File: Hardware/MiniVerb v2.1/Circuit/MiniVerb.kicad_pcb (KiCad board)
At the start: 2 copper layers, 47.9 x 128.5 mm, 52 parts, among them J1 IDC_2x05, U1 TL074, U2 LM4040DBZ-10, U3 MCP6001-OT

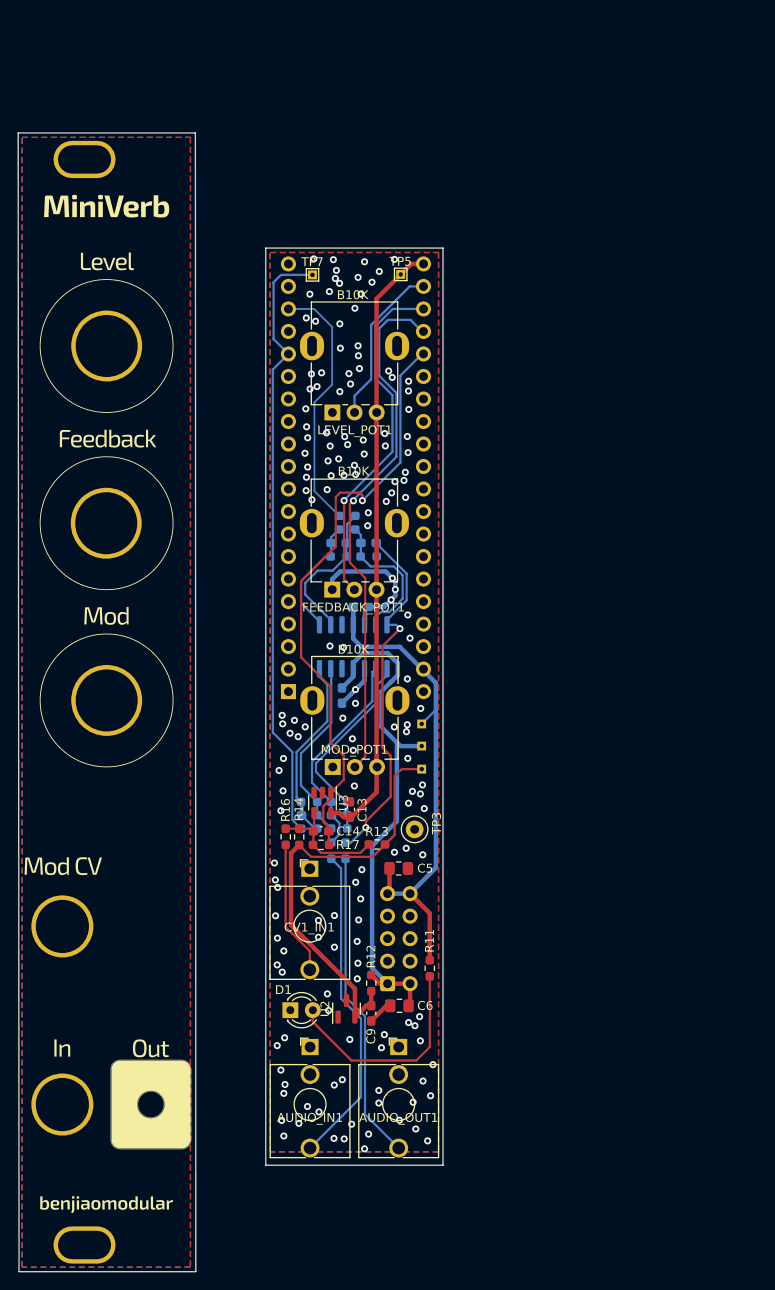
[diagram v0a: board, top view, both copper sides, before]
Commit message: cleanup and ibom
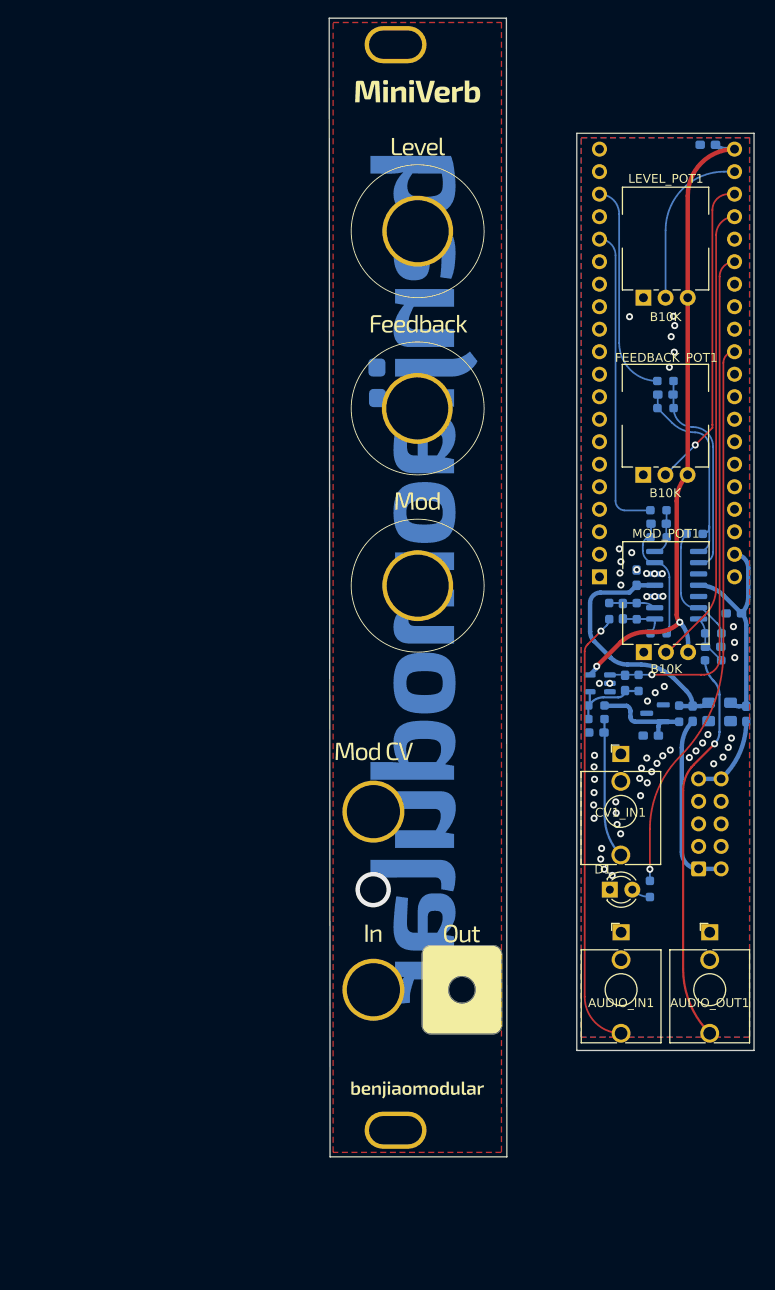
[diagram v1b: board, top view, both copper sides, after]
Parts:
- removed R14: 200k, Resistor_SMD:R_0603_1608Metric_Pad0.98x0.95mm_HandSolder
- removed TP1: TP_12V, TestPoint:TestPoint_THTPad_1.0x1.0mm_Drill0.5mm
- removed TP2: TP_-12V, TestPoint:TestPoint_THTPad_1.0x1.0mm_Drill0.5mm
- removed TP3: TP_GND, TestPoint:TestPoint_Loop_D1.80mm_Drill1.0mm_Beaded
- removed TP4: TP_-10V, TestPoint:TestPoint_THTPad_1.0x1.0mm_Drill0.5mm
- removed TP5: TP_3.3V, TestPoint:TestPoint_THTPad_1.0x1.0mm_Drill0.5mm
- removed TP7: TP_INPUT_BUFFER, TestPoint:TestPoint_THTPad_1.0x1.0mm_Drill0.5mm
- added C10: 100nF, Capacitor_SMD:C_0603_1608Metric_Pad1.08x0.95mm_HandSolder, B.Cu at (162.3, 117.7)
- added FB1: 742792664, Capacitor_SMD:C_0603_1608Metric_Pad1.08x0.95mm_HandSolder, B.Cu at (179.2, 115.6)
- added FB2: 742792664, Capacitor_SMD:C_0603_1608Metric_Pad1.08x0.95mm_HandSolder, B.Cu at (173.2, 115.5)
- C13, C5, C6, C9, R12, R13, R16, U2, U3: moved to B.Cu
- C14: value 4.7nF -> 10nF; moved to B.Cu
- FEEDBACK_POT1, LEVEL_POT1, MOD_POT1: footprint benjiaomodular:Potentiometer_RV09 -> benjiaomodular:Potentiometer_RV09_NoBracket
- R11: value 10k -> 220; moved to B.Cu
- R17: value 33k -> 66.5k; moved to B.Cu
- moved C13 85.2 mm to (174.9, 51.3), turned to 180 degrees
- moved R10 53.3 mm to (169.3, 92.6)
- moved C3 51.4 mm to (169.3, 94.1), turned to 180 degrees
- moved R7 49.5 mm to (169.3, 95.6), turned to 180 degrees
- moved U2 48.2 mm to (168.9, 115.5), turned to 180 degrees
- moved C6 48.1 mm to (175.0, 115.3), turned to 90 degrees
- moved R9 46.7 mm to (175.5, 109.5), turned to 0 degrees
- moved R12 46.2 mm to (171.6, 115.5)
- moved C9 44.5 mm to (168.4, 118.0), turned to 180 degrees
- moved R5 42.2 mm to (169.3, 106.5), turned to 180 degrees
- moved C7 42.1 mm to (177.8, 104.2), turned to 180 degrees
- moved C5 41.4 mm to (177.4, 115.3), turned to -90 degrees
- moved R2 41.4 mm to (163.8, 104.0)
- moved C4 40.6 mm to (175.5, 108.0), turned to 0 degrees
- moved R3 40.5 mm to (170.1, 81.1)
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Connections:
- A1 pad 25: CV1 -> unconnected-(A1-Pad25)
- A1 pad 26: unconnected-(A1-Pad26) -> CV1
- A1 pad 30: unconnected-(A1-Pad30) -> LED
- J1 pad 1: -12V -> Net-(FB2-Pad1)
- J1 pad 10: +12V -> Net-(FB1-Pad1)
- J1 pad 2: -12V -> Net-(FB2-Pad1)
- J1 pad 9: +12V -> Net-(FB1-Pad1)
- R11 pad 2: +12V -> LED
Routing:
- net LED: track 0.00 -> 62.5 mm, vias 0 -> 1
- net AREF_-10: track 49.2 -> 11.6 mm
- net Net-(C4-Pad1): track 41.9 -> 5.19 mm, vias 2 -> 0
- net INT_AUDIO_IN1: track 69.1 -> 35.0 mm
- net +12V: track 56.1 -> 26.1 mm
- net -12V: track 59.2 -> 30.4 mm
- net GND: track 24.3 -> 0.00 mm, vias 157 -> 57
- net Net-(D1-Pad2): track 24.9 -> 2.20 mm
- net Net-(FB2-Pad1): track 0.00 -> 20.5 mm
- net Net-(C2-Pad2): track 24.2 -> 5.27 mm
- net Net-(C2-Pad1): track 22.9 -> 5.34 mm
- net Net-(C3-Pad1): track 21.0 -> 5.29 mm
- net Net-(AUDIO_IN1-PadT): track 36.4 -> 50.0 mm, vias 0 -> 1
- net Net-(FB1-Pad1): track 0.00 -> 9.76 mm
- net Net-(AUDIO_OUT1-PadT): track 35.1 -> 44.7 mm, vias 0 -> 1
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- removed copper zone on B.Cu, net (none)
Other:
- outline, holes or cut-outs redrawn
